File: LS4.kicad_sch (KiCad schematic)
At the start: 3 parts, among them U7 VNLD5160TR-E

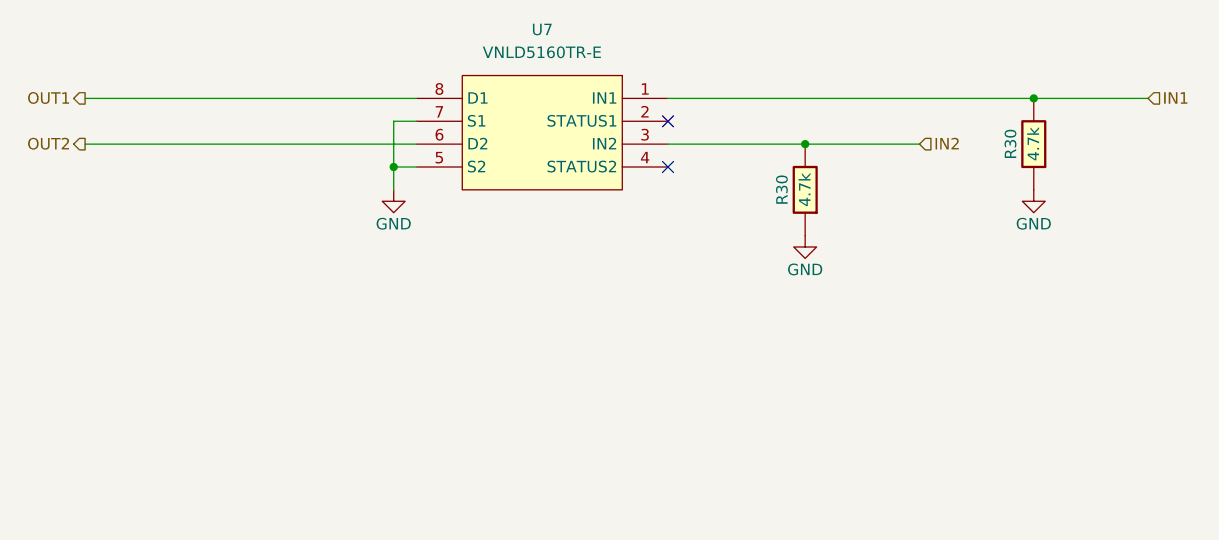
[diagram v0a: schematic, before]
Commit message: reset
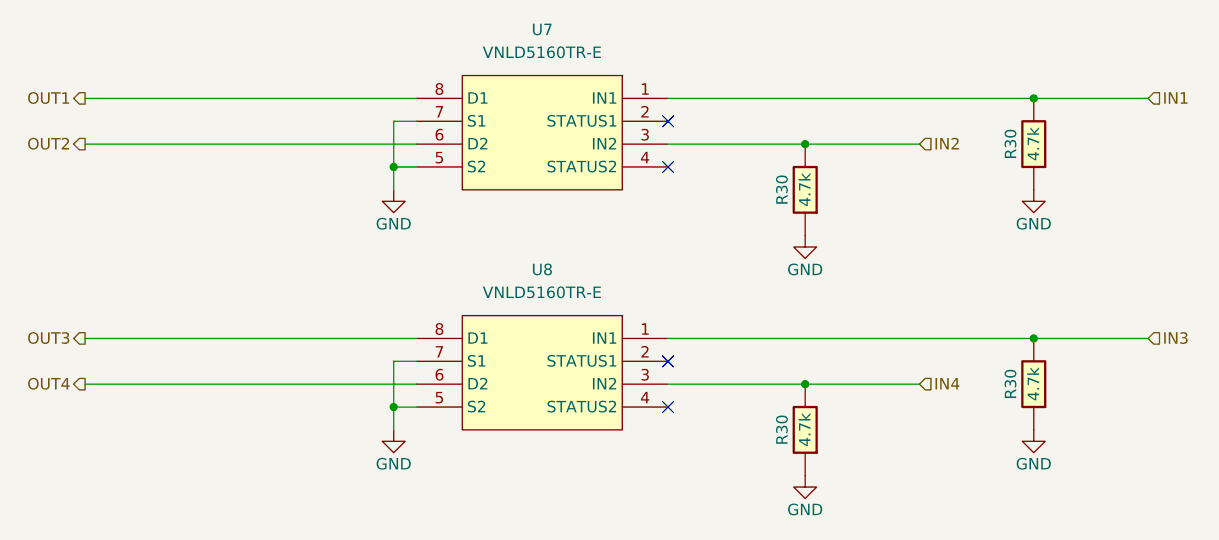
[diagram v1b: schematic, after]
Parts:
- added R30 (x2): 4.7k, hellen-one-common:R0603, symbol hellen-one-common:Res
- added U8: VNLD5160TR-E, Package_SO:SOIC-8_3.9x4.9mm_P1.27mm, symbol chips:VNLD5160
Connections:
- net GND: now also R30.1, R30.1, U8.5 (S2), U8.7 (S1)
- new net IN3: R30.2, U8.1 (IN1)
- new net IN4: R30.2, U8.3 (IN2)
- new net OUT3: U8.8 (D1)
- new net OUT4: U8.6 (D2)
- no-connect marks 2 -> 4
